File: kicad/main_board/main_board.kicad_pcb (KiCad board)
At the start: 2 copper layers, 160 x 80 mm, 114 parts, among them J1 2.54mm PinHeader 1x03 Male, J10 Micro_SD_Card, J11 2.54mm PinHeader 1x03 Male, J12 Conn_ARM_JTAG_SWD_10, J13 JST-PH 1x02 Male, J2 JST-PH 1x03 Male, J3 Barrel_Jack, J4 JST-PH 1x02 Male, J5 JST-PH 1x02 Male, J6 JST-PH 1x02 Male, J7 JST-PH 1x03 Male, J8 2.54mm PinHeader 1x03 Male, J9 JST-PH 1x03 Male, Q1 PN2222A, Q2 BD139, Q3 BD139, Q4 PN2222A, SW1 SW_Push, SW2 SW_Push, U1 AZ1117-3.3, U2 Amazon_Small_Buck, U3 ESP32-WROOM-32

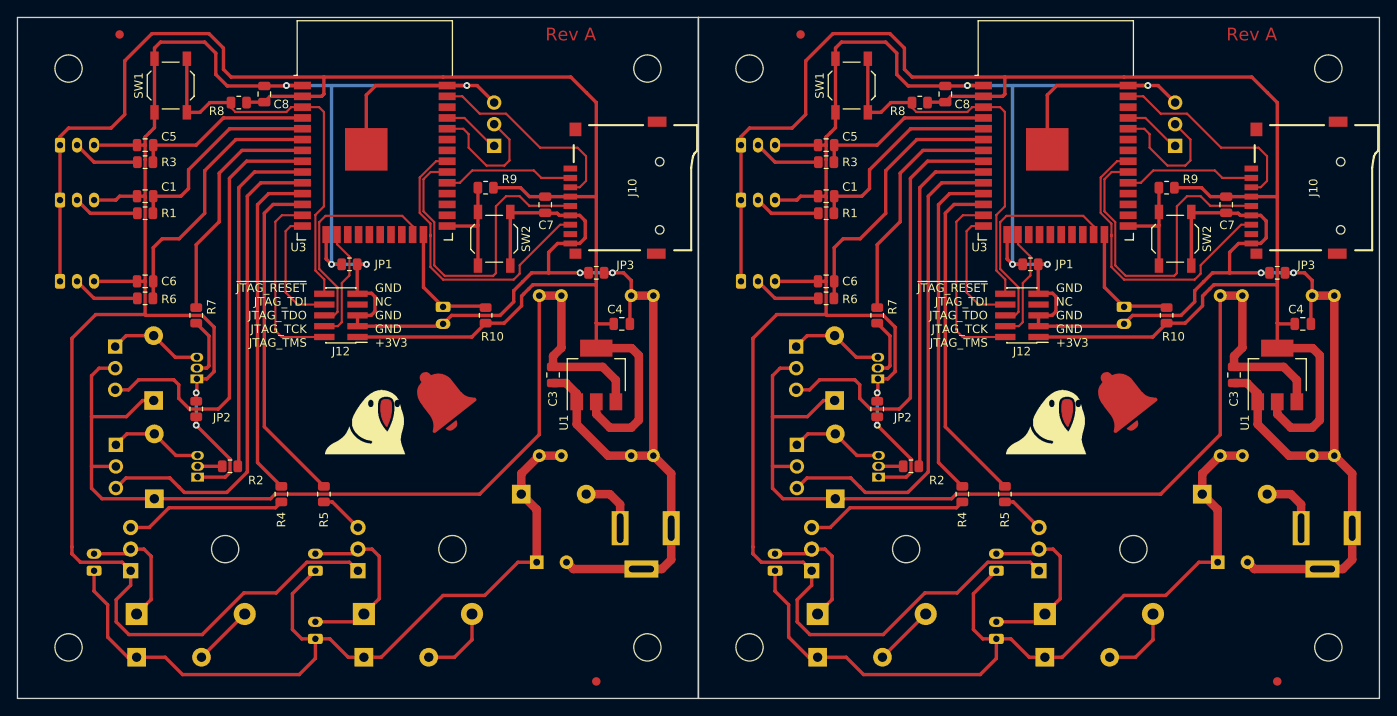
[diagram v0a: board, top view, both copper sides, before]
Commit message: Upload old changes
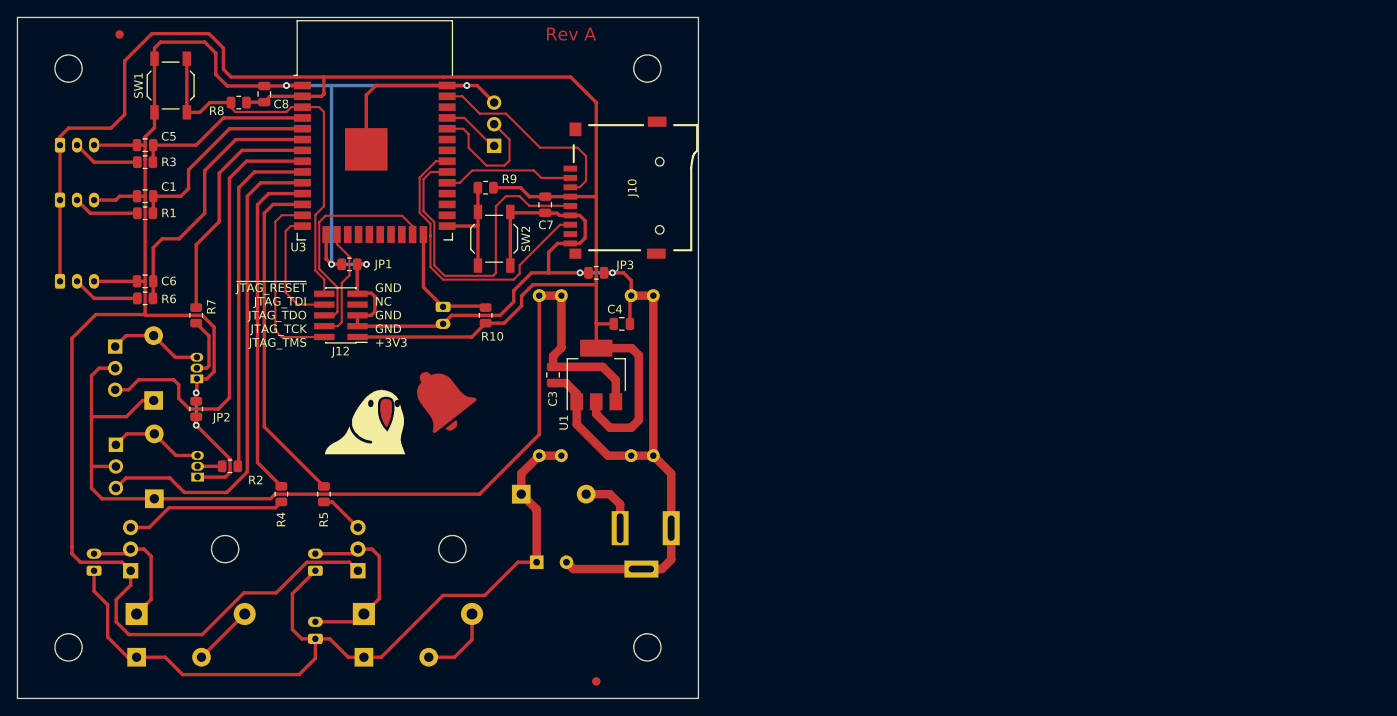
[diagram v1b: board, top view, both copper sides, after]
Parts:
- removed the C1 at (119.0, 42.0)
- removed the C2 at (165.0, 85.0)
- removed the C3 at (166.9, 63.0)
- removed the C4 at (175.0, 57.0)
- removed the C5 at (119.0, 36.0)
- removed the C6 at (119.0, 52.0)
- removed the C7 at (166.0, 43.0)
- removed the C8 at (133.0, 30.0)
- removed the D1 at (163.2, 77.0)
- removed the D2 at (120.1, 77.5)
- removed the D3 at (118.0, 96.2)
- removed the D4 at (144.7, 96.2)
- removed the D5 at (118.0, 91.1)
- removed the D6 at (144.7, 91.1)
- removed the D7 at (120.0, 66.0)
- removed the GRAPHIC1 at (149.0, 67.0)
- removed the GRAPHIC2 at (116.0, 23.0)
- removed the GRAPHIC3 at (172.0, 99.0)
- removed the H1 at (110.0, 95.0)
- removed the H2 at (110.0, 27.0)
- removed the H3 at (178.0, 27.0)
- removed the H4 at (178.0, 95.0)
- removed the J1 at (115.6, 71.2)
- removed the J10 at (168.2, 41.0)
- removed the J11 at (160.0, 36.1)
- removed the J12 at (142.0, 56.0)
- removed the J13 at (154.0, 55.0)
- removed the J2 at (109.0, 42.5)
- removed the J3 at (188.3, 81.0)
- removed the J4 at (113.0, 86.0)
- removed the J5 at (139.0, 94.0)
- removed the J6 at (139.0, 86.0)
- removed the J7 at (109.0, 36.0)
- removed the J8 at (115.5, 59.7)
- removed the J9 at (109.0, 52.0)
- removed the JP1 at (143.0, 50.0)
- removed the JP2 at (125.0, 67.0)
- removed the JP3 at (172.0, 51.0)
- removed the Q1 at (125.2, 75.0)
- removed the Q2 at (117.3, 86.0)
- removed the Q3 at (144.0, 86.0)
- removed the Q4 at (125.1, 63.5)
- removed the R1 at (119.0, 44.0)
- removed the R10 at (159.0, 56.0)
- removed the R2 at (129.0, 73.7)
- removed the R3 at (119.0, 38.0)
- removed the R4 at (135.0, 77.0)
- removed the R5 at (140.0, 77.0)
- removed the R6 at (119.0, 54.0)
- removed the R7 at (125.0, 56.0)
- removed the R8 at (130.0, 31.0)
- removed the R9 at (159.0, 41.0)
- removed the SW1 at (122.0, 29.0)
- removed the SW2 at (160.0, 47.0)
- removed the U1 at (172.0, 63.0)
- removed the U2 at (172.0, 63.1)
- removed the U3 at (146.0, 37.2)
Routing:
- net GND: track 815.4 -> 407.7 mm, vias 16 -> 8
- net +3V3: track 400.7 -> 200.3 mm
- net +5V: track 243.7 -> 121.8 mm
- net +12V: track 194.4 -> 97.2 mm
- net /LEFT_SERVO_PULSE: track 114.3 -> 57.2 mm
- net /RIGHT_SERVO_PULSE: track 104.0 -> 52.0 mm
- net /~{JTAG_RESET}: track 92.7 -> 46.4 mm
- net /LEFT_SERVO_ENABLE: track 82.0 -> 41.0 mm
- net /BELL_ENABLE: track 80.1 -> 40.1 mm
- net /LIGHT_ENABLE: track 79.8 -> 39.9 mm
- net /VSPI_SCLK: track 78.4 -> 39.2 mm
- net /VSPI_MISO: track 71.1 -> 35.6 mm
- net /LIGHT_DIMMER_POS: track 63.4 -> 31.7 mm
- net /RIGHT_SERVO_ENABLE: track 55.6 -> 27.8 mm
- net /JTAG_TDO: track 51.9 -> 25.9 mm
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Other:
- board size 160 x 80 mm -> 80 x 80 mm
